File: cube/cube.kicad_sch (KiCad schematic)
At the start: 87 parts, among them Q1 Q_NPN_BCE, Q2 Q_NPN_BCE, Q3 Q_NPN_BCE, Q4 Q_NPN_BCE, Q5 Q_NPN_BCE, Q6 Q_NPN_BCE, Q7 Q_NPN_BCE, Q8 Q_NPN_BCE, SW1 SW_Push, U1 74HC595, U2 74HC595, U3 74HC595, U4 74HC595, U5 74HC595, U6 74HC595, U7 74HC595, U8 74HC595, U9 74HC595

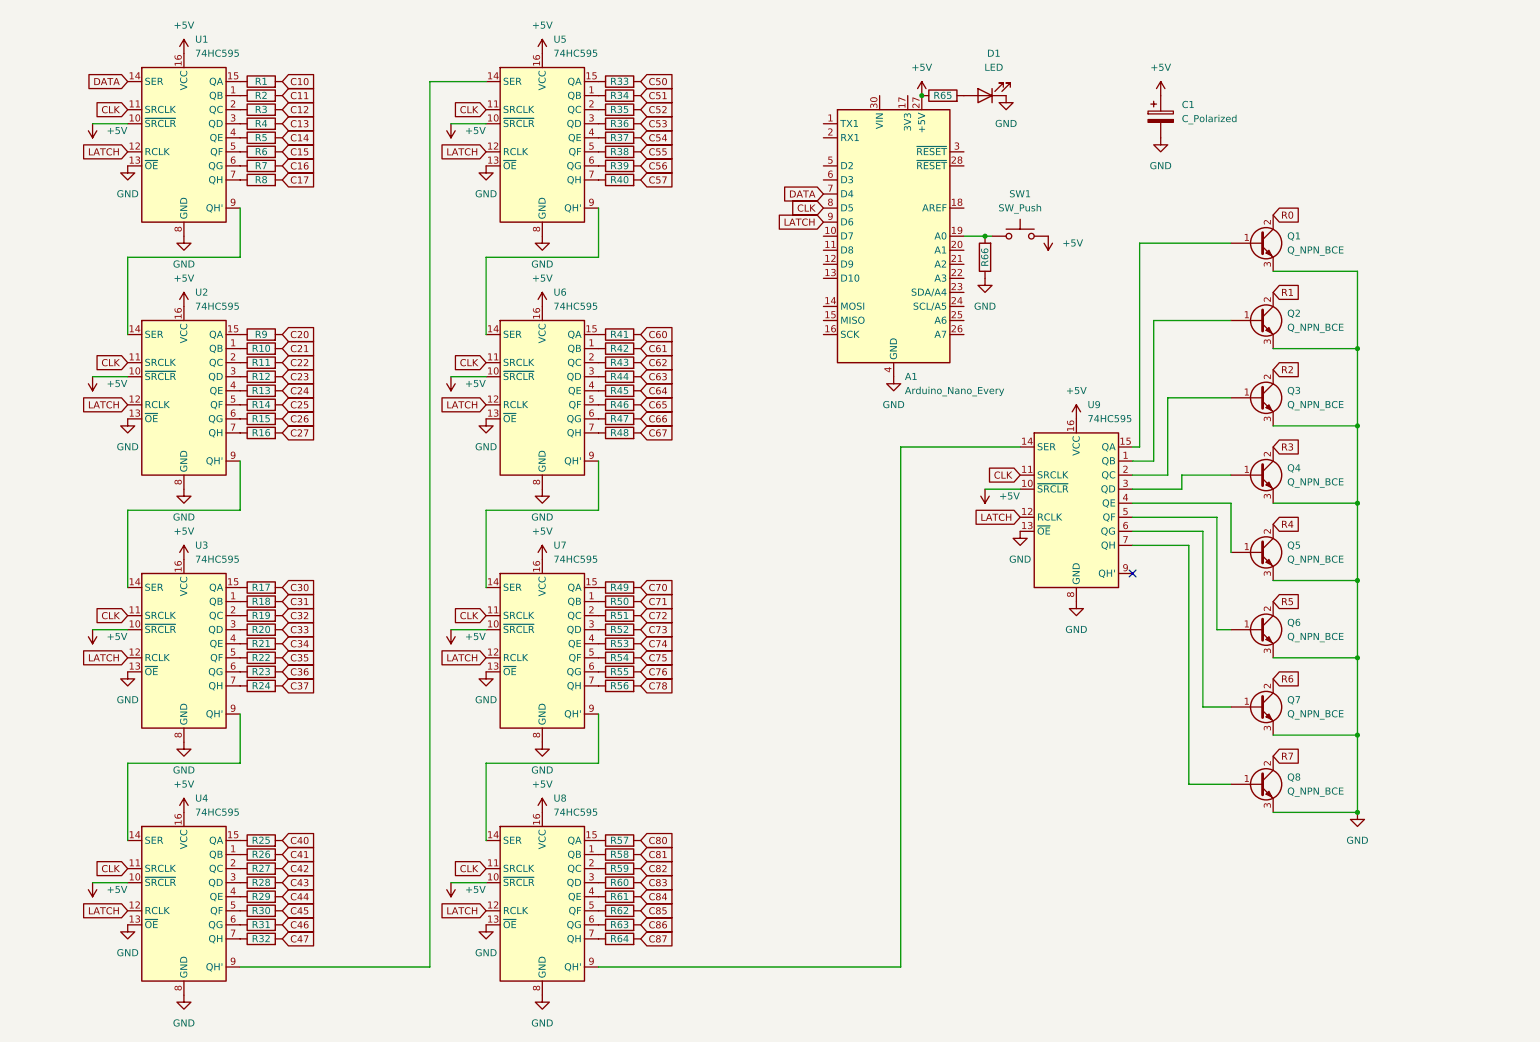
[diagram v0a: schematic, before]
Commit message: created pcb
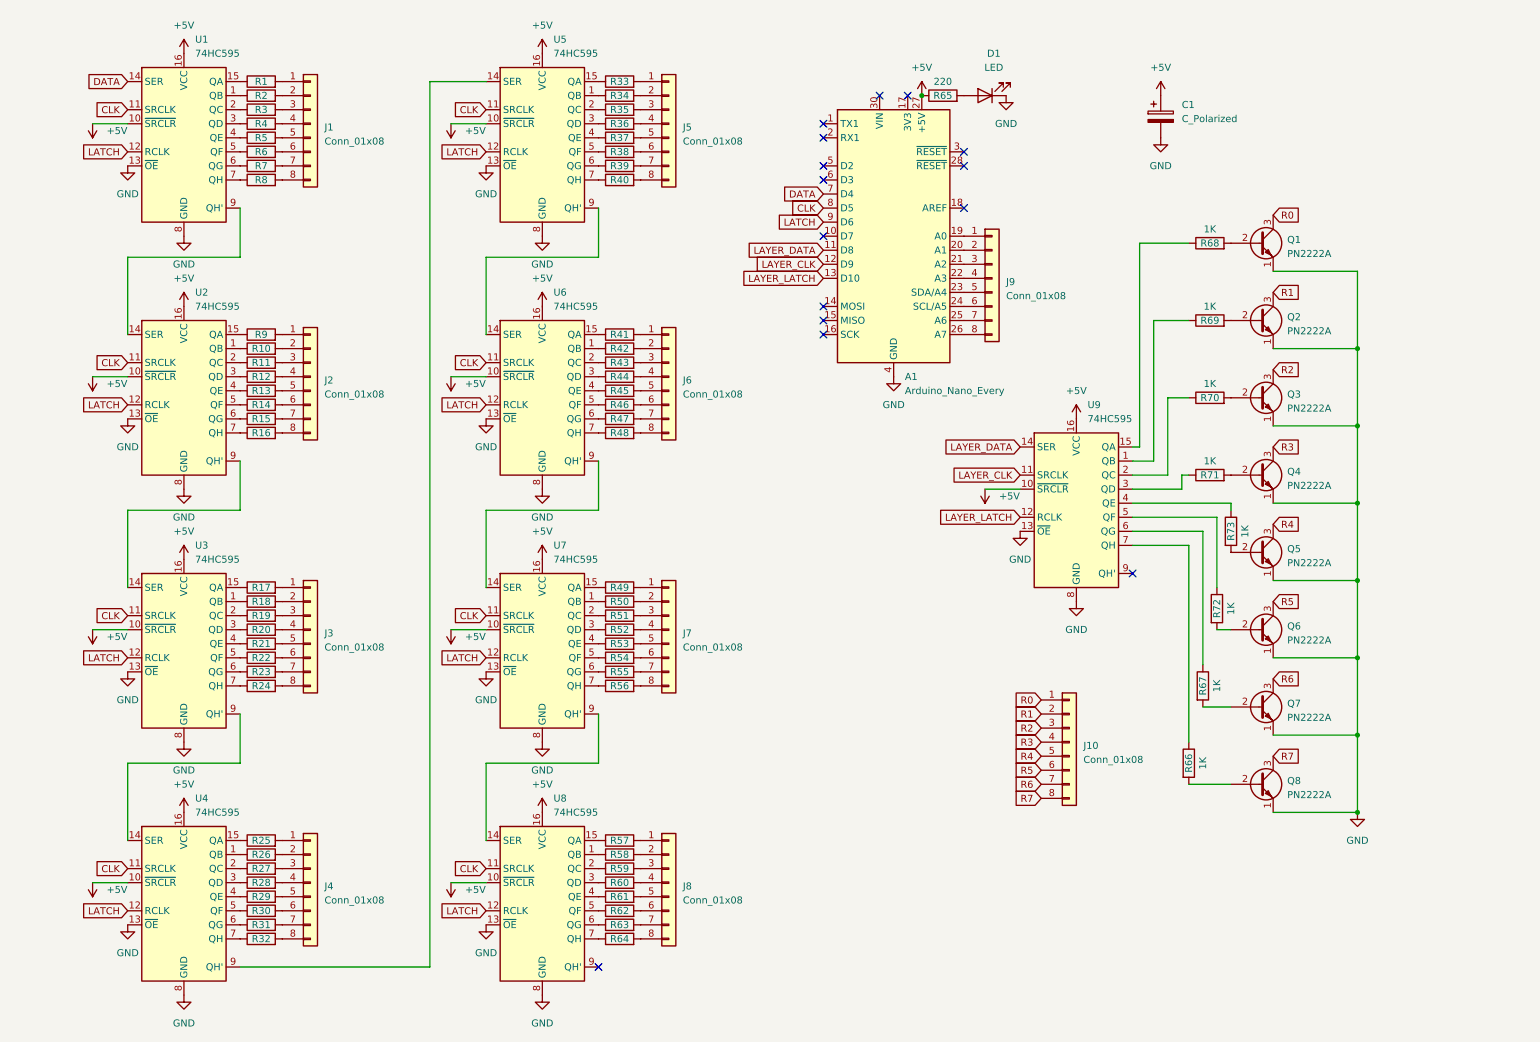
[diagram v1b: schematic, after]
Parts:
- removed Q1, Q2, Q3, Q4, Q5, Q6, Q7, Q8: Q_NPN_BCE, symbol Device:Q_NPN_BCE
- removed SW1: SW_Push, symbol Switch:SW_Push
- added J1, J10, J2, J3, J4, J5, J6, J7, J8, J9: Conn_01x08, Connector_PinHeader_2.54mm:PinHeader_1x08_P2.54mm_Vertical, symbol Connector_Generic:Conn_01x08
- added Q1, Q2, Q3, Q4, Q5, Q6, Q7, Q8: PN2222A, Package_TO_SOT_THT:TO-92_Inline, symbol Transistor_BJT:PN2222A
- added R67, R68, R69, R70, R71, R72, R73: 1K, Resistor_THT:R_Axial_DIN0207_L6.3mm_D2.5mm_P10.16mm_Horizontal, symbol Device:R
- C1: footprint (none) -> Capacitor_THT:C_Radial_D10.0mm_H20.0mm_P5.00mm
- D1: footprint (none) -> LED_THT:LED_D5.0mm_Clear
- R1, R10, R11, R12, R13, R14, R15, R16, R17, R18, R19, R2, R20, R21, R22, R23, R24, R25, R26, R27, R28, R29, R3, R30, R31, R32, R33, R34, R35, R36, R37, R38, R39, R4, R40, R41, R42, R43, R44, R45, R46, R47, R48, R49, R5, R50, R51, R52, R53, R54, R55, R56, R57, R58, R59, R6, R60, R61, R62, R63, R64, R7, R8, R9: footprint (none) -> Resistor_THT:R_Axial_DIN0207_L6.3mm_D2.5mm_P10.16mm_Horizontal
- R65: value R -> 220; footprint (none) -> Resistor_THT:R_Axial_DIN0207_L6.3mm_D2.5mm_P10.16mm_Horizontal
- R66: value R -> 1K; footprint (none) -> Resistor_THT:R_Axial_DIN0207_L6.3mm_D2.5mm_P10.16mm_Horizontal
- U1, U2, U3, U4, U5, U6, U7, U8, U9: footprint (none) -> Package_DIP:DIP-16_W7.62mm_Socket
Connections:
- net CLK: no longer U9.11 (SRCLK)
- net GND: now also Q1.1 (E), Q2.1 (E), Q3.1 (E), Q4.1 (E), Q5.1 (E), Q6.1 (E), Q7.1 (E), Q8.1 (E); no longer R66.1
- net LATCH: no longer U9.12 (RCLK)
- net R0: now also J10.1 (Pin_1), Q1.3 (C)
- net R1: now also J10.2 (Pin_2), Q2.3 (C)
- net R2: now also J10.3 (Pin_3), Q3.3 (C)
- net R3: now also J10.4 (Pin_4), Q4.3 (C)
- net R4: now also J10.5 (Pin_5), Q5.3 (C)
- net R5: now also J10.6 (Pin_6), Q6.3 (C)
- net R6: now also J10.7 (Pin_7), Q7.3 (C)
- net R7: now also J10.8 (Pin_8), Q8.3 (C)
- net at U9.3 (QD): now also R71.1
- net at U9.5 (QF): now also R72.1
- net at R66.2: now also Q8.2 (B); no longer A1.19 (A0)
- net at U9.6 (QG): now also R67.1
- net LAYER_DATA: now reaches A1.11 (D8)
- net LAYER_DATA: now also U9.14 (SER)
- net LAYER_CLK: now reaches A1.12 (D9)
- net LAYER_CLK: now also U9.11 (SRCLK)
- net LAYER_LATCH: now reaches A1.13 (D10)
- net LAYER_LATCH: now also U9.12 (RCLK)
- net at A1.20 (A1): now also J9.2 (Pin_2)
- net at A1.21 (A2): now also J9.3 (Pin_3)
- net at A1.22 (A3): now also J9.4 (Pin_4)
- net at A1.23 (SDA/A4): now also J9.5 (Pin_5)
- net at A1.24 (SCL/A5): now also J9.6 (Pin_6)
- net at A1.25 (A6): now also J9.7 (Pin_7)
- net at A1.26 (A7): now also J9.8 (Pin_8)
- net at U9.1 (QB): now also R69.1
- net at U8.9 (QH'): no longer U9.14 (SER)
- net at U9.15 (QA): now also R68.1
- net at U9.2 (QC): now also R70.1
- net at U9.4 (QE): now also R73.1
- net at U9.7 (QH): now also R66.1
- net C10: no longer names the net of R1.2
- net C10: now also J1.1 (Pin_1)
- net C11: no longer names the net of R2.2
- net C11: now also J1.2 (Pin_2)
- net C12: no longer names the net of R3.2
- net C12: now also J1.3 (Pin_3)
- net C13: no longer names the net of R4.2
- net C13: now also J1.4 (Pin_4)
- net C14: no longer names the net of R5.2
- net C14: now also J1.5 (Pin_5)
- net C15: no longer names the net of R6.2
- net C15: now also J1.6 (Pin_6)
- net C16: no longer names the net of R7.2
- net C16: now also J1.7 (Pin_7)
- net C17: no longer names the net of R8.2
- net C17: now also J1.8 (Pin_8)
- net C20: no longer names the net of R9.2
- net C20: now also J2.1 (Pin_1)
- net C21: no longer names the net of R10.2
- net C21: now also J2.2 (Pin_2)
- net C22: no longer names the net of R11.2
- net C22: now also J2.3 (Pin_3)
- net C23: no longer names the net of R12.2
- net C23: now also J2.4 (Pin_4)
- net C24: no longer names the net of R13.2
- net C24: now also J2.5 (Pin_5)
- net C25: no longer names the net of R14.2
- net C25: now also J2.6 (Pin_6)
- net C26: no longer names the net of R15.2
- net C26: now also J2.7 (Pin_7)
- net C27: no longer names the net of R16.2
- net C27: now also J2.8 (Pin_8)
- net C30: no longer names the net of R17.2
- net C30: now also J3.1 (Pin_1)
- net C31: no longer names the net of R18.2
- net C31: now also J3.2 (Pin_2)
- net C32: no longer names the net of R19.2
- net C32: now also J3.3 (Pin_3)
- net C33: no longer names the net of R20.2
- net C33: now also J3.4 (Pin_4)
- net C34: no longer names the net of R21.2
- net C34: now also J3.5 (Pin_5)
- net C35: no longer names the net of R22.2
- net C35: now also J3.6 (Pin_6)
- net C36: no longer names the net of R23.2
- net C36: now also J3.7 (Pin_7)
- net C37: no longer names the net of R24.2
- net C37: now also J3.8 (Pin_8)
- net C40: no longer names the net of R25.2
- net C40: now also J4.1 (Pin_1)
- net C41: no longer names the net of R26.2
- net C41: now also J4.2 (Pin_2)
- net C42: no longer names the net of R27.2
- net C42: now also J4.3 (Pin_3)
- net C43: no longer names the net of R28.2
- net C43: now also J4.4 (Pin_4)
- net C44: no longer names the net of R29.2
- net C44: now also J4.5 (Pin_5)
- net C45: no longer names the net of R30.2
- net C45: now also J4.6 (Pin_6)
- net C46: no longer names the net of R31.2
- net C46: now also J4.7 (Pin_7)
- net C47: no longer names the net of R32.2
- net C47: now also J4.8 (Pin_8)
- net C50: no longer names the net of R33.2
- net C50: now also J5.1 (Pin_1)
- net C51: no longer names the net of R34.2
- net C51: now also J5.2 (Pin_2)
- net C52: no longer names the net of R35.2
- net C52: now also J5.3 (Pin_3)
- net C53: no longer names the net of R36.2
- net C53: now also J5.4 (Pin_4)
- net C54: no longer names the net of R37.2
- net C54: now also J5.5 (Pin_5)
- net C55: no longer names the net of R38.2
- net C55: now also J5.6 (Pin_6)
- net C56: no longer names the net of R39.2
- net C56: now also J5.7 (Pin_7)
- net C57: no longer names the net of R40.2
- net C57: now also J5.8 (Pin_8)
- net C60: no longer names the net of R41.2
- net C60: now also J6.1 (Pin_1)
- net C61: no longer names the net of R42.2
- net C61: now also J6.2 (Pin_2)
- net C62: no longer names the net of R43.2
- net C62: now also J6.3 (Pin_3)
- net C63: no longer names the net of R44.2
- net C63: now also J6.4 (Pin_4)
- net C64: no longer names the net of R45.2
- net C64: now also J6.5 (Pin_5)
- net C65: no longer names the net of R46.2
- net C65: now also J6.6 (Pin_6)
- net C66: no longer names the net of R47.2
- net C66: now also J6.7 (Pin_7)
- net C67: no longer names the net of R48.2
- net C67: now also J6.8 (Pin_8)
- net C70: no longer names the net of R49.2
- net C70: now also J7.1 (Pin_1)
- net C71: no longer names the net of R50.2
- net C71: now also J7.2 (Pin_2)
- net C72: no longer names the net of R51.2
- net C72: now also J7.3 (Pin_3)
- net C73: no longer names the net of R52.2
- net C73: now also J7.4 (Pin_4)
- net C74: no longer names the net of R53.2
- net C74: now also J7.5 (Pin_5)
- net C75: no longer names the net of R54.2
- net C75: now also J7.6 (Pin_6)
- net C76: no longer names the net of R55.2
- net C76: now also J7.7 (Pin_7)
- net C78: no longer names the net of R56.2
- net C78: now also J7.8 (Pin_8)
- net C80: no longer names the net of R57.2
- net C80: now also J8.1 (Pin_1)
- net C81: no longer names the net of R58.2
- net C81: now also J8.2 (Pin_2)
- net C82: no longer names the net of R59.2
- net C82: now also J8.3 (Pin_3)
- net C83: no longer names the net of R60.2
- net C83: now also J8.4 (Pin_4)
- net C84: no longer names the net of R61.2
- net C84: now also J8.5 (Pin_5)
- net C85: no longer names the net of R62.2
- net C85: now also J8.6 (Pin_6)
- net C86: no longer names the net of R63.2
- net C86: now also J8.7 (Pin_7)
- net C87: no longer names the net of R64.2
- net C87: now also J8.8 (Pin_8)
- new net: Q2.2 (B), R69.2
- new net: Q5.2 (B), R73.2
- new net: Q6.2 (B), R72.2
- new net: Q1.2 (B), R68.2
- new net: A1.19 (A0), J9.1 (Pin_1)
- new net: Q3.2 (B), R70.2
- new net: Q7.2 (B), R67.2
- new net: Q4.2 (B), R71.2
- no-connect marks 1 -> 15

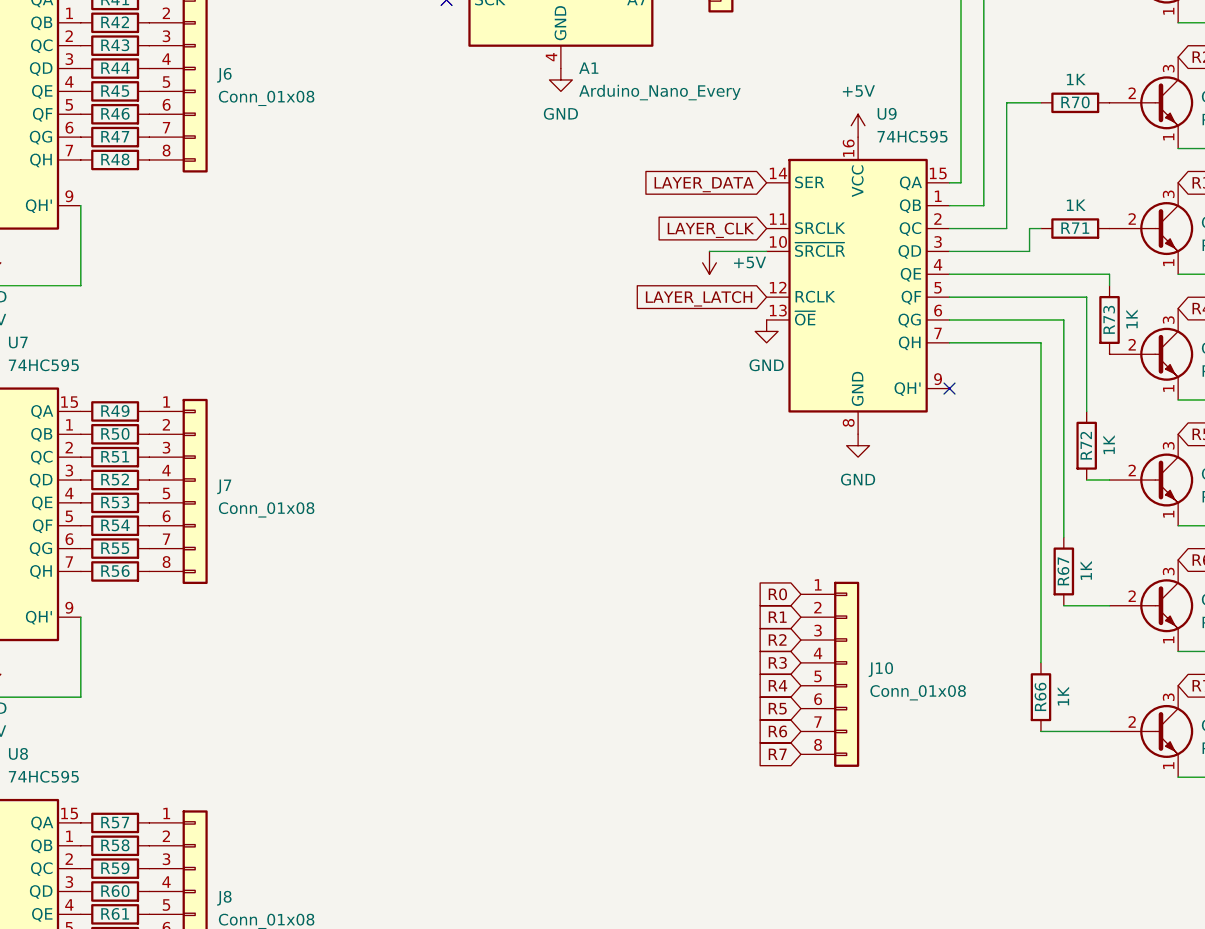
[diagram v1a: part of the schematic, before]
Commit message: updated pcb.
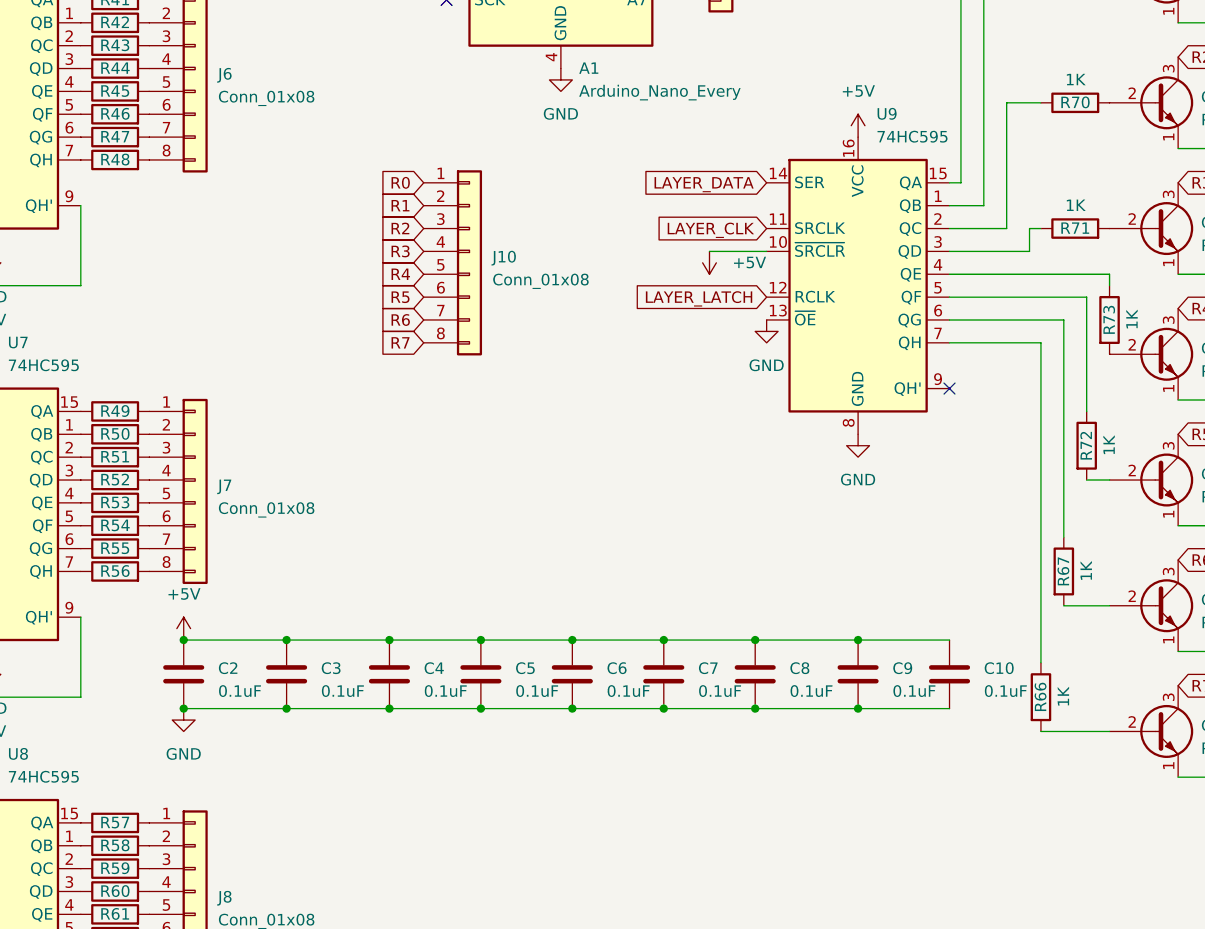
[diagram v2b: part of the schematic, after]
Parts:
- added C10, C2, C3, C4, C5, C6, C7, C8, C9: 0.1uF, Capacitor_THT:C_Disc_D5.1mm_W3.2mm_P5.00mm, symbol Device:C
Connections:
- net +5V: now also C10.1, C2.1, C3.1, C4.1, C5.1, C6.1, C7.1, C8.1, C9.1
- net GND: now also C10.2, C2.2, C3.2, C4.2, C5.2, C6.2, C7.2, C8.2, C9.2
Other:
- moved on the sheet: J10
